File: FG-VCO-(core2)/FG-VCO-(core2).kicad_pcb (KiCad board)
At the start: 2 copper layers, 53.3 x 106.7 mm, 59 parts, among them J1 main_power, J11 Test Saw, J14 conn_power, J2 conn_signals_1, J3 conn_signals_2, J4 Test Ramp, J5 Test Triangle, J6 Test Sine, J7 Test Square, J8 conn_signals_3, Q2 2N7000, U1 74LS73, U10 74LS169, U11 74LS169, U3 TL074, U4 TL082, U6 DAC08, U7 DAC08, U8 74HC590

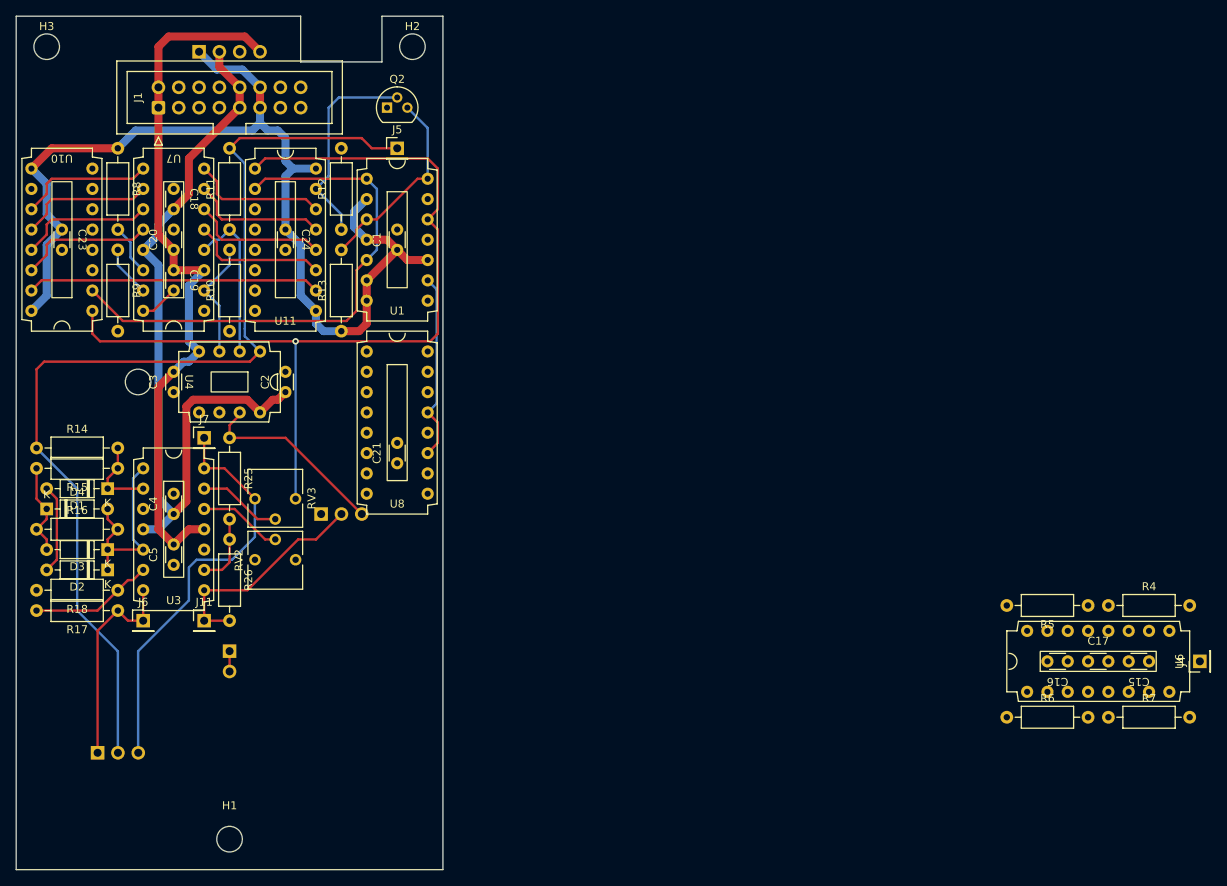
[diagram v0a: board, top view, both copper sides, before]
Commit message: same as previous, for the whole folder
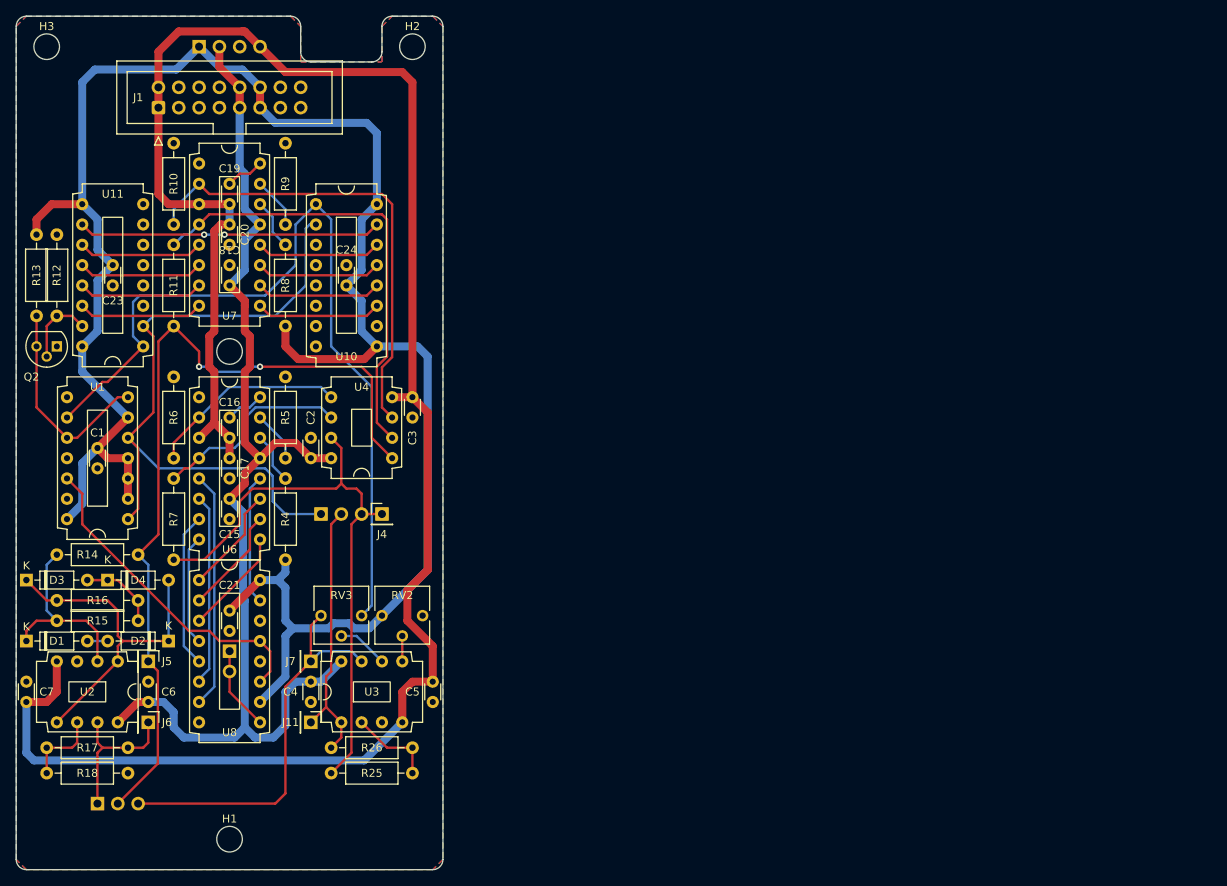
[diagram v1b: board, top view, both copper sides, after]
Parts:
- added C6: 4n7, Custom Footprints:C_Disc_P2.54mm, F.Cu at (16.5, 84.5)
- added C7: 4n7, Custom Footprints:C_Disc_P2.54mm, F.Cu at (1.27, 84.5)
- added U2: TL082, Custom Footprints:DIP-8_central_caps, F.Cu at (8.89, 84.5)
- U3: value TL074 -> TL082; footprint Custom Footprints:DIP-14_central_caps -> Custom Footprints:DIP-8_central_caps
- moved R7 120.6 mm to (19.7, 57.8), turned to -90 degrees
- moved C15 115.3 mm to (26.7, 61.6), turned to 90 degrees
- moved R6 112.5 mm to (19.7, 45.1), turned to -90 degrees
- moved C17 111.2 mm to (26.7, 56.5), turned to -90 degrees
- moved U6 111.2 mm to (26.7, 56.5), turned to 0 degrees
- moved C16 107.5 mm to (26.7, 51.4), turned to 90 degrees
- moved R4 104.1 mm to (33.7, 57.8), turned to -90 degrees
- moved J4 103.9 mm to (45.7, 62.2), turned to 0 degrees
- moved R5 102.0 mm to (33.7, 55.2), turned to 90 degrees
- moved J5 71.3 mm to (16.5, 80.6), turned to -90 degrees
- moved Q2 50.9 mm to (5.08, 41.3), turned to 180 degrees
- moved C1 46.4 mm to (10.2, 55.2), turned to -90 degrees
- moved U1 46.4 mm to (10.2, 55.2), turned to 180 degrees
- moved R25 43.8 mm to (39.4, 94.6), turned to 0 degrees
- moved R13 40.0 mm to (2.54, 27.3), turned to -90 degrees
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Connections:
- U1 pad 10: +5V -> /Flip-Flops/RCO
- U1 pad 12: /Flip-Flops/U/D -> /Flip-Flops/f_clk/2
- U1 pad 14: /Flip-Flops/RCO -> +5V
- U1 pad 3: /Flip-Flops/RCO -> +5V
- U1 pad 7: +5V -> /Flip-Flops/RCO
- U1 pad 9: /Flip-Flops/f_clk/2 -> /Flip-Flops/U/D
- U3 pad 1: Net-(D2-Pad1) -> Saw
- U3 pad 2: Net-(D1-Pad1) -> Net-(R25-Pad2)
- U3 pad 4: +12V -> -12V
- U3 pad 5: Net-(D2-Pad1) -> Net-(RV2-Pad2)
- U3 pad 6: Net-(R17-Pad2) -> Net-(RV3-Pad2)
- U3 pad 7: Sine -> Square
- U3 pad 8: Saw -> +12V
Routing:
- net -12V: track 90.0 -> 252.4 mm
- net +5V: track 131.1 -> 253.1 mm
- net Ramp: track 23.9 -> 74.9 mm
- net +12V: track 98.6 -> 143.1 mm
- net Net-(R10-Pad2): track 14.8 -> 59.3 mm
- net Net-(R11-Pad1): track 20.0 -> 57.1 mm
- net /Digital Analog Converter Ramp/QR7: track 0.00 -> 29.5 mm
- net Net-(R7-Pad1): track 0.00 -> 25.3 mm
- net Triangle: track 130.0 -> 104.9 mm, vias 0 -> 2
- net Net-(R6-Pad2): track 0.00 -> 25.0 mm
- net /Digital Analog Converter Ramp/QR6: track 0.00 -> 23.9 mm
- net f_clk: track 67.7 -> 88.0 mm
- net Net-(D2-Pad1): track 24.3 -> 44.0 mm
- net /Digital Analog Converter Ramp/QR5: track 0.00 -> 19.4 mm
- net /Flip-Flops/f_clk/2: track 23.6 -> 40.9 mm
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- added copper zone on B.Cu, net GNDD
- added copper zone on F.Cu, net GNDD
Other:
- outline, holes or cut-outs redrawn
